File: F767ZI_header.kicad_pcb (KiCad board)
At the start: 2 copper layers, 73 x 98.4 mm, 22 parts, among them J2 CAN1, J3 CAN2, J4 UART, J5 PowerBoard, J6 EMERSW_CON, J7 I2C1_default, J9 RESET_SW, SW1 SW_Push, U1 MCP2562-E-P, U2 MCP2562-E-P

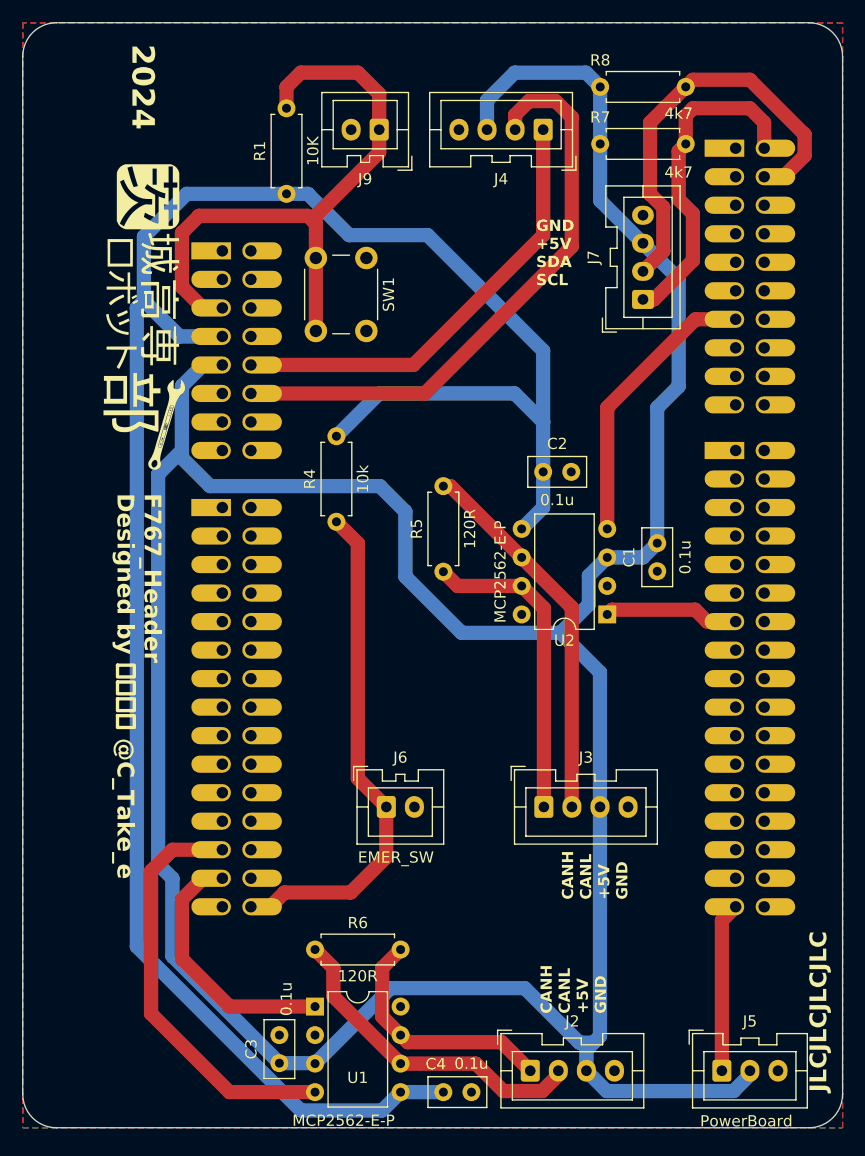
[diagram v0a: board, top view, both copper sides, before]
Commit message: PCB: 部品密度こそ正義
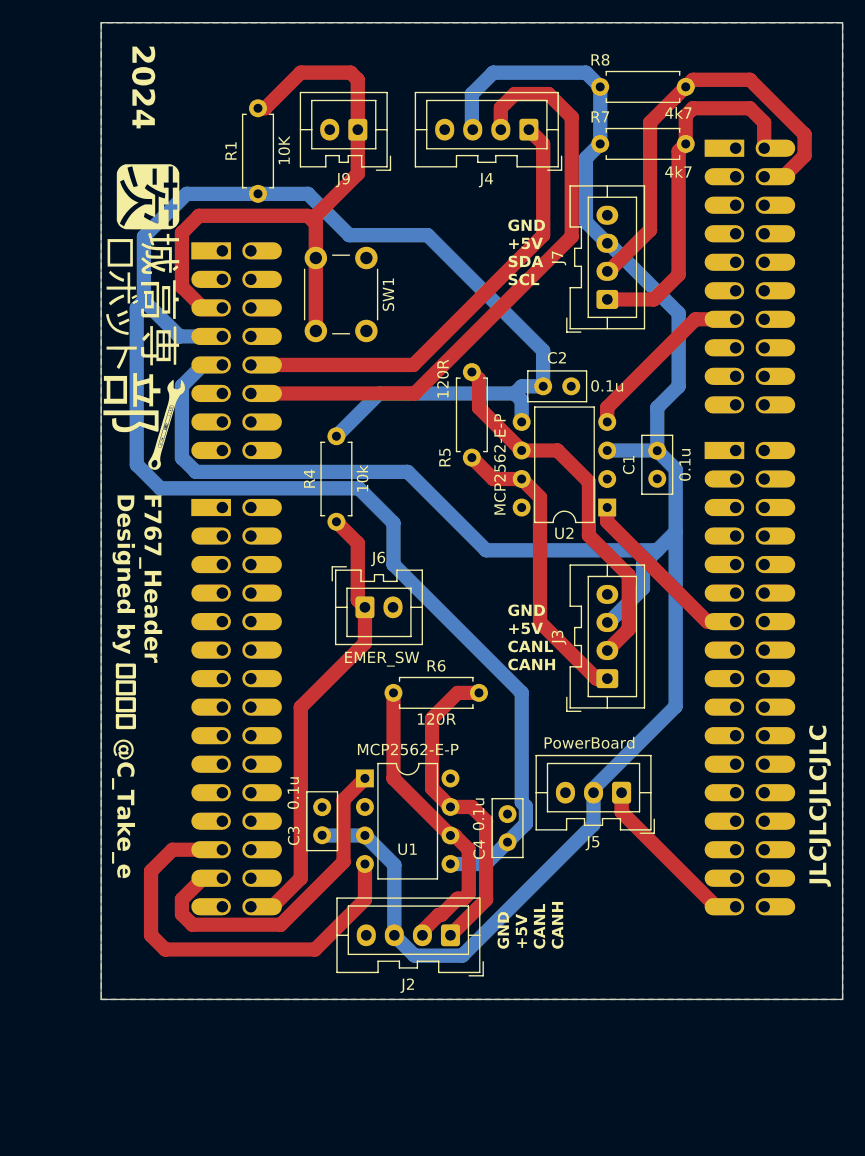
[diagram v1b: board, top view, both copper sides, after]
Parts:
- moved J5 26.3 mm to (207.6, 118.7), turned to 180 degrees
- moved R6 23.9 mm to (194.9, 109.9)
- moved C4 23.0 mm to (197.5, 123.2), turned to 90 degrees
- moved U1 20.8 mm to (184.8, 117.5)
- moved C3 20.7 mm to (181.0, 122.5)
- moved J6 17.9 mm to (184.8, 102.2)
- moved J2 14.0 mm to (192.4, 131.4), turned to 180 degrees
- moved J3 12.8 mm to (206.4, 108.6), turned to 90 degrees
- moved R5 10.5 mm to (194.3, 88.9)
- moved U2 9.53 mm to (206.4, 93.3)
- moved C1 8.23 mm to (210.8, 88.3)
- moved C2 7.62 mm to (200.7, 82.5)
- moved J7 3.18 mm to (206.4, 74.8)
- moved R1 2.54 mm to (175.3, 57.8)
- moved J9 1.91 mm to (184.2, 59.7)
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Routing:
- net +5V: track 278.0 -> 200.7 mm
- net +3V3: track 186.5 -> 162.9 mm
- net CAN2_RD: track 25.5 -> 16.0 mm
- net CAN1_TD: track 23.3 -> 31.0 mm
- net CAN1H: track 21.8 -> 28.9 mm
- net EMER_SW: track 45.6 -> 40.7 mm
- net CAN2_TD: track 12.1 -> 16.4 mm
- net CAN1L: track 29.3 -> 26.8 mm
- net I2C1_SCL: track 29.7 -> 31.8 mm
- net UART_RX: track 53.0 -> 54.6 mm
- net CAN2H: track 28.0 -> 26.7 mm
- net UART_TX: track 40.2 -> 40.7 mm
- net NRST: track 56.9 -> 56.4 mm
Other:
- board size 73 x 98.4 mm -> 66 x 87 mm
- board text added: "GND +5V CANL CANH"
- board text removed: "CANH CANL +5V GND"
